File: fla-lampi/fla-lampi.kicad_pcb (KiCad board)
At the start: 2 copper layers, 24 x 34 mm, 6 parts, among them J1 Screw_Terminal_01x03_P3.5mm, M1 Module_XIAO-RP2040_SocketSMD, SW1 BUTTON_B3SN, SW2 BUTTON_B3SN

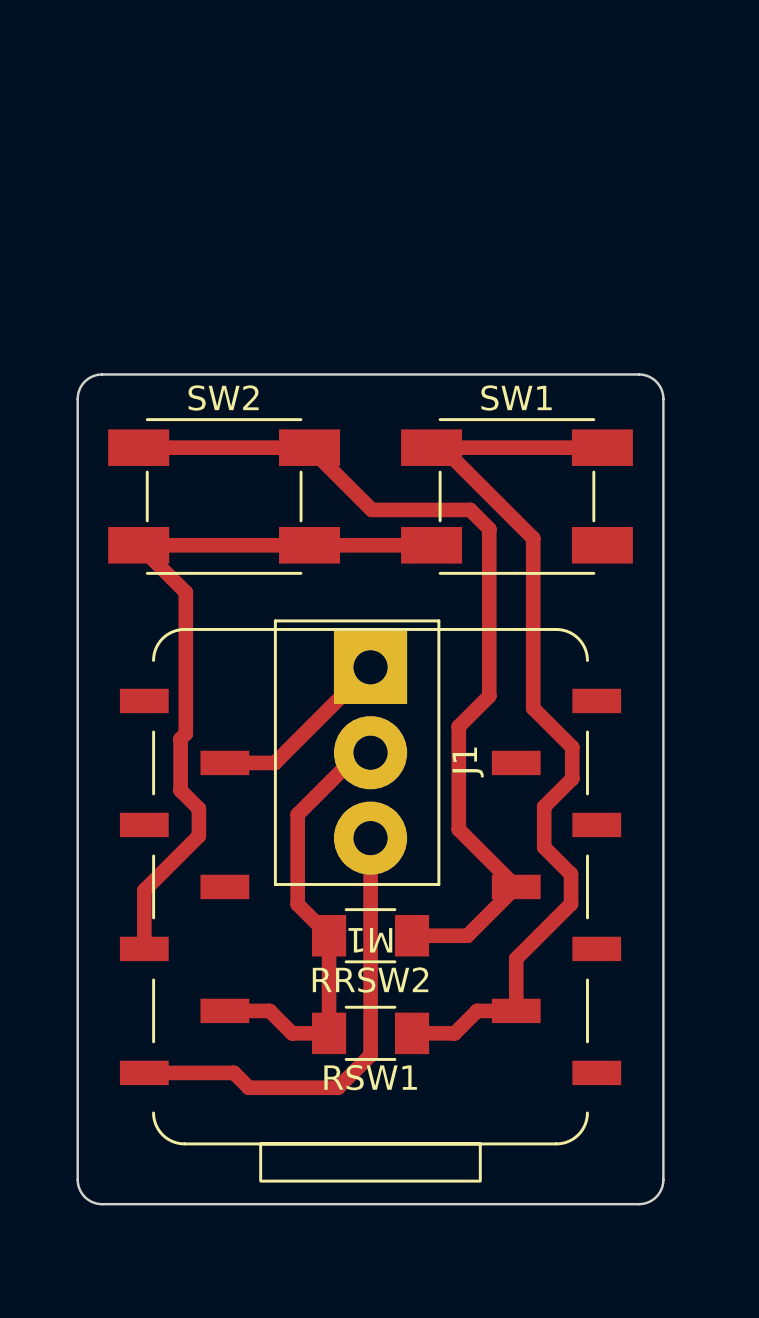
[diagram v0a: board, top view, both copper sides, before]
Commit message: Bretti
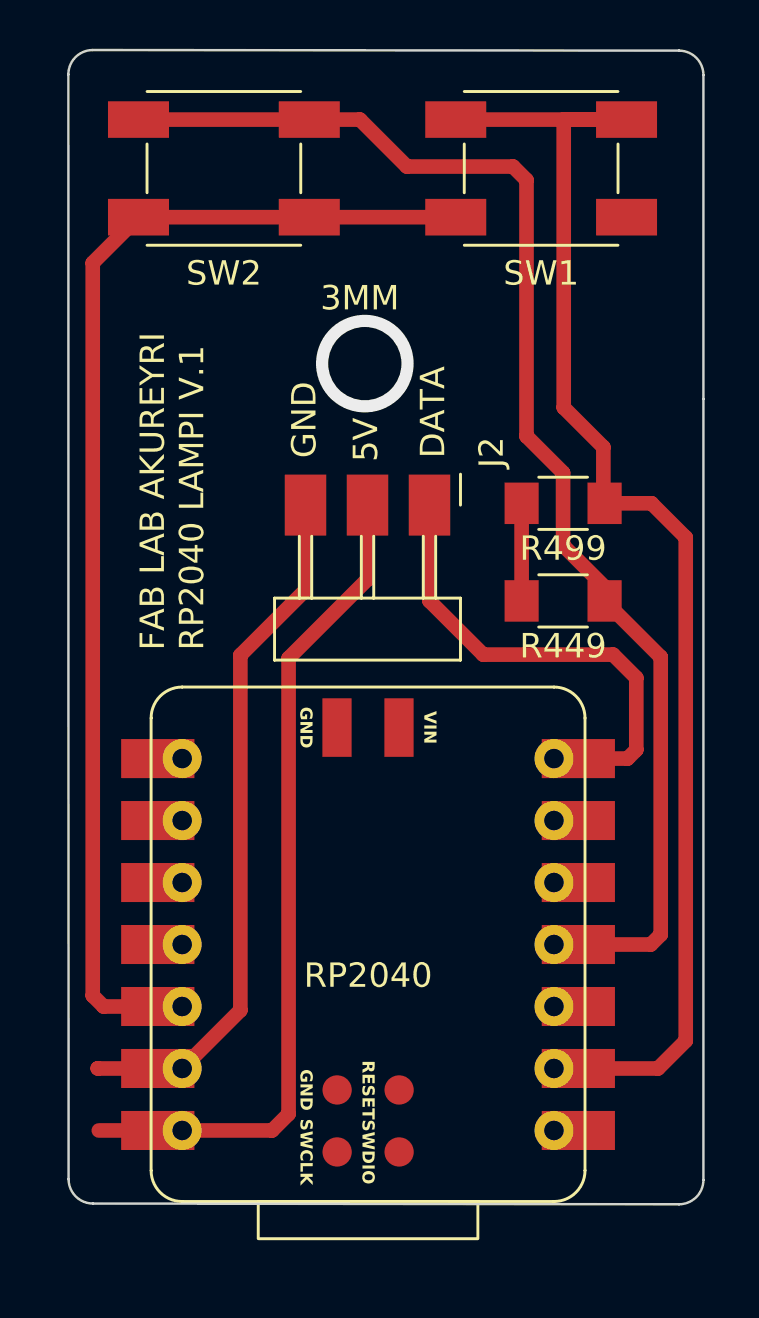
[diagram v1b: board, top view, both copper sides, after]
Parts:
- removed J1: Screw_Terminal_01x03_P3.5mm, fab:TerminalBlock_OnShore_1x03_P3.50mm_Horizontal
- removed M1: Module_XIAO-RP2040_SocketSMD, fab:SeeedStudio_XIAO_SocketSMD
- added J2: Conn_PinHeader_1x03_P2.54mm_Horizontal_SMD, fab:PinHeader_1x03_P2.54mm_Horizontal_SMD, F.Cu at (154.6, 121.5)
- added RP2040: Module_XIAO-RP2040, fab:SeeedStudio_XIAO_RP2040, F.Cu at (152.0, 139.5)
- moved R499 23.1 mm to (160.0, 121.5)
- moved R449 15.8 mm to (160.0, 125.5)
- moved SW1 13.5 mm to (159.1, 107.7)
- moved SW2 13.4 mm to (146.1, 107.7)
- renumbered RRSW2 to R449, RSW1 to R499
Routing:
- net A6: track 0.01 -> 20.2 mm
- net PWR_3V3: track 30.7 -> 49.5 mm
- net A3: track 37.0 -> 54.7 mm
- net A1: track 39.2 -> 56.4 mm
- net PWR_5V: track 19.0 -> 34.3 mm
- net GND: track 18.2 -> 32.7 mm
- net A8: track 7.59 -> 0.00 mm
- net (no net): vias 0 -> 1
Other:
- board size 24 x 34 mm -> 26 x 47.3 mm
- board text added: "3MM"
- board text added: "5V"
- board text added: "DATA"
- board text added: "FAB LAB AKUREYRI RP2040 LAMPI V.1"
- board text added: "GND"

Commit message: Update pinout and project
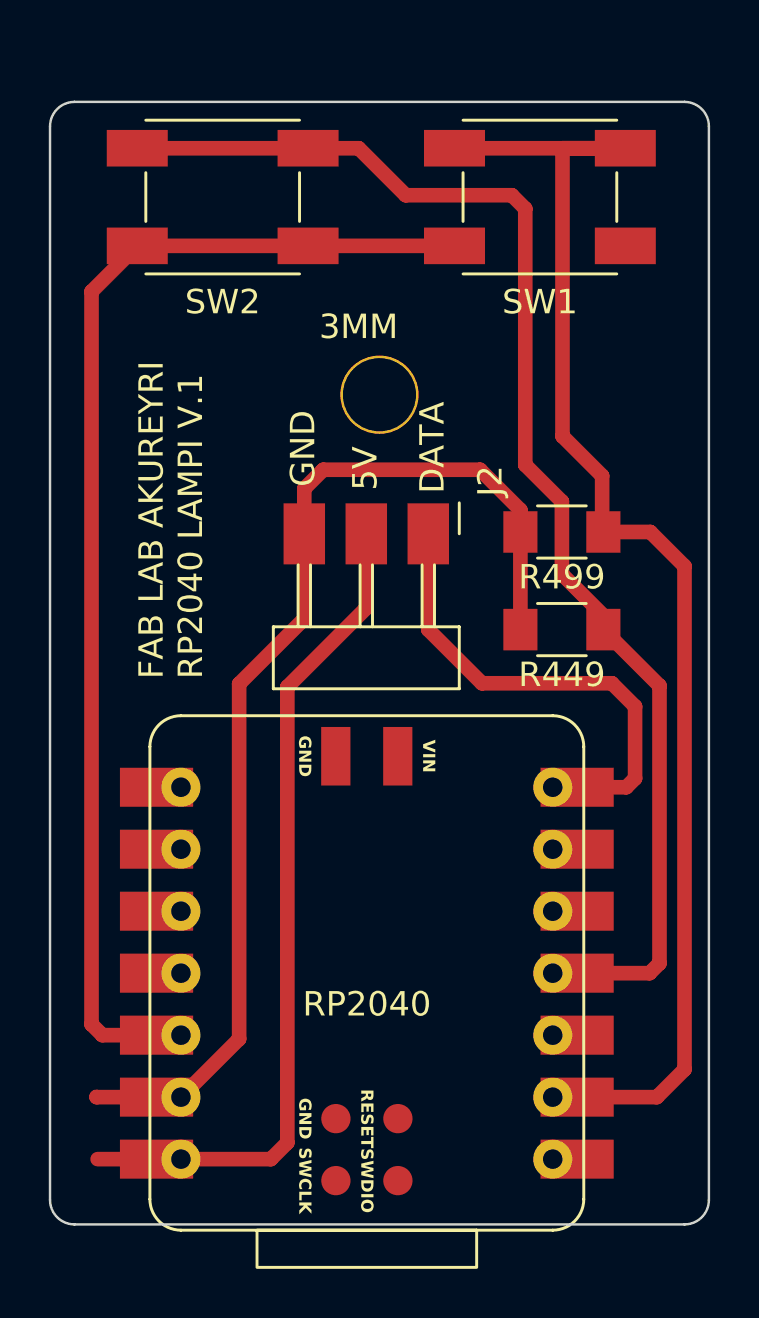
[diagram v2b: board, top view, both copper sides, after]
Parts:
- added REF**: MountingHole_3mm, fab:MountingHole_3mm, F.Cu at (152.5, 117.0)
- moved RP2040 1.18 mm to (152.0, 140.7)
- moved J2 1.18 mm to (154.5, 122.7)
- moved R449 1.18 mm to (160.0, 126.6)
- moved R499 1.18 mm to (160.0, 122.6)
- moved SW1 1.18 mm to (159.1, 108.9)
- moved SW2 1.18 mm to (146.1, 108.9)
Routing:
- net GND: track 32.7 -> 45.3 mm
- net (no net): vias 1 -> 0
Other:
- board size 26 x 47.3 mm -> 27 x 46 mm
